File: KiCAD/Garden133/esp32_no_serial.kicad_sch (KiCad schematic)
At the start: 13 parts, among them J1 USB_B_Micro, J2 Edge2x6_Connector, U3 ESP32-WROOM-32, U4 NCP114ASN330T1G

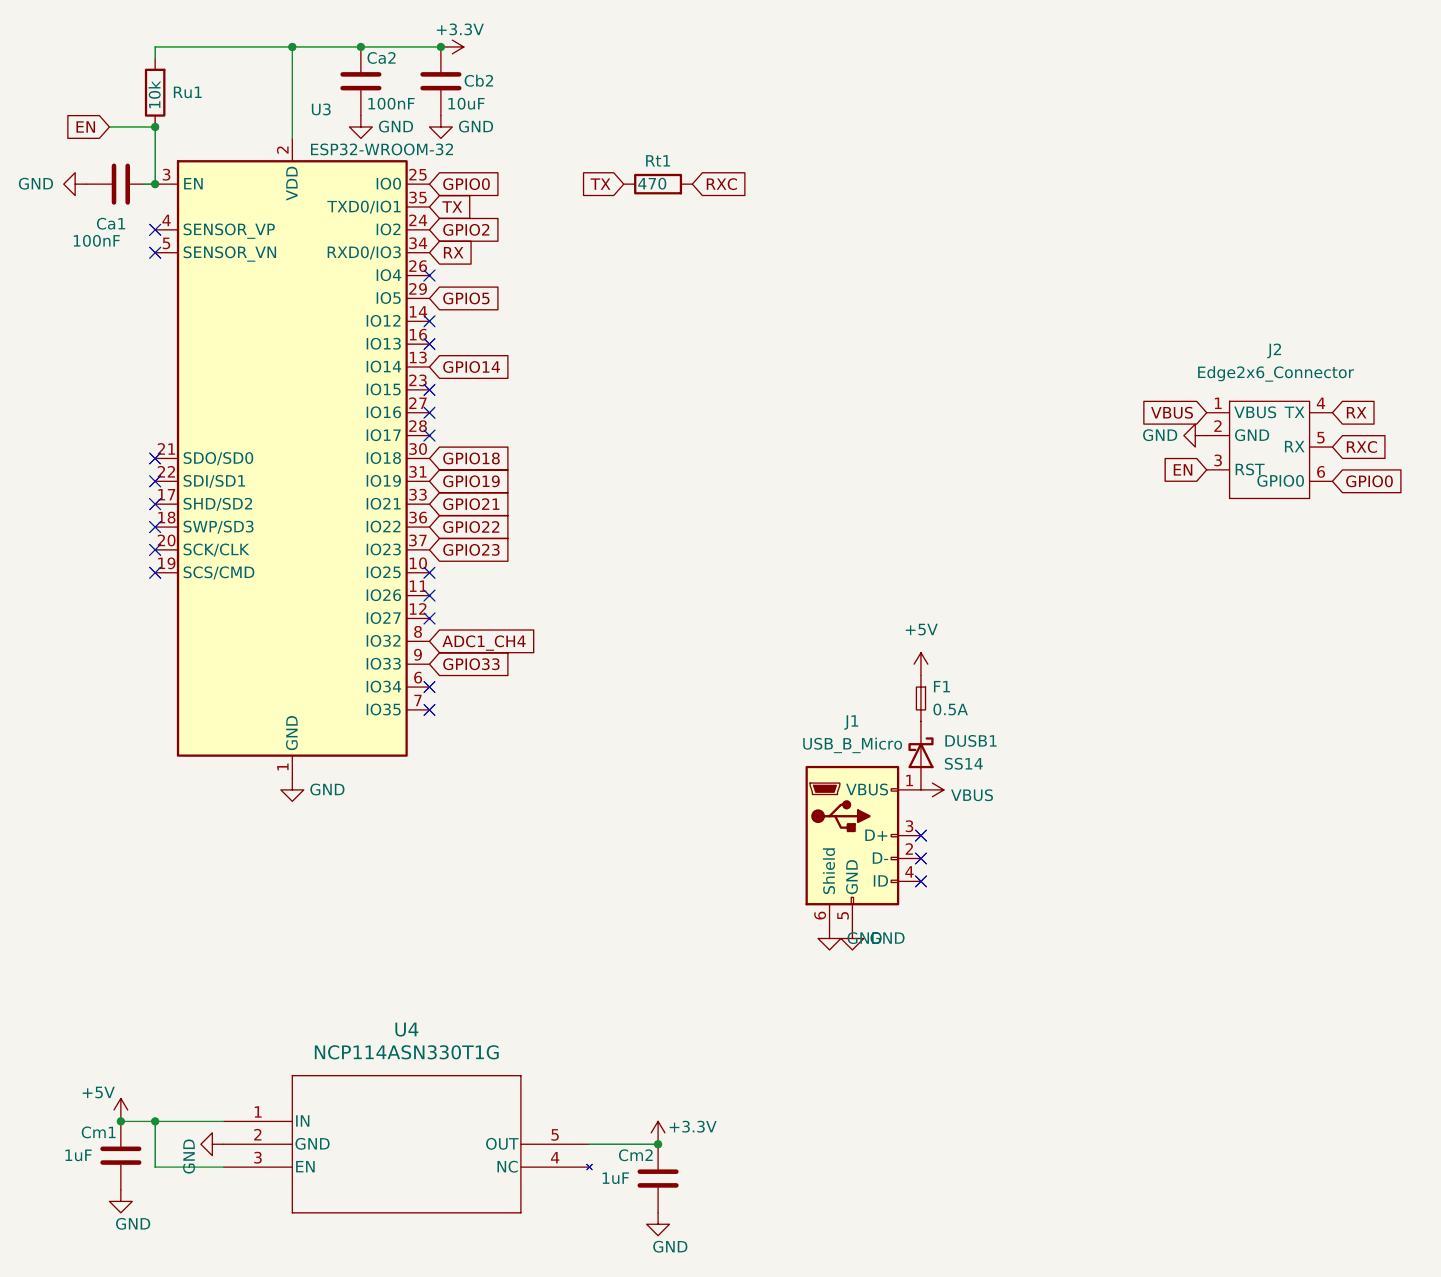
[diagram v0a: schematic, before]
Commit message: Board version 5
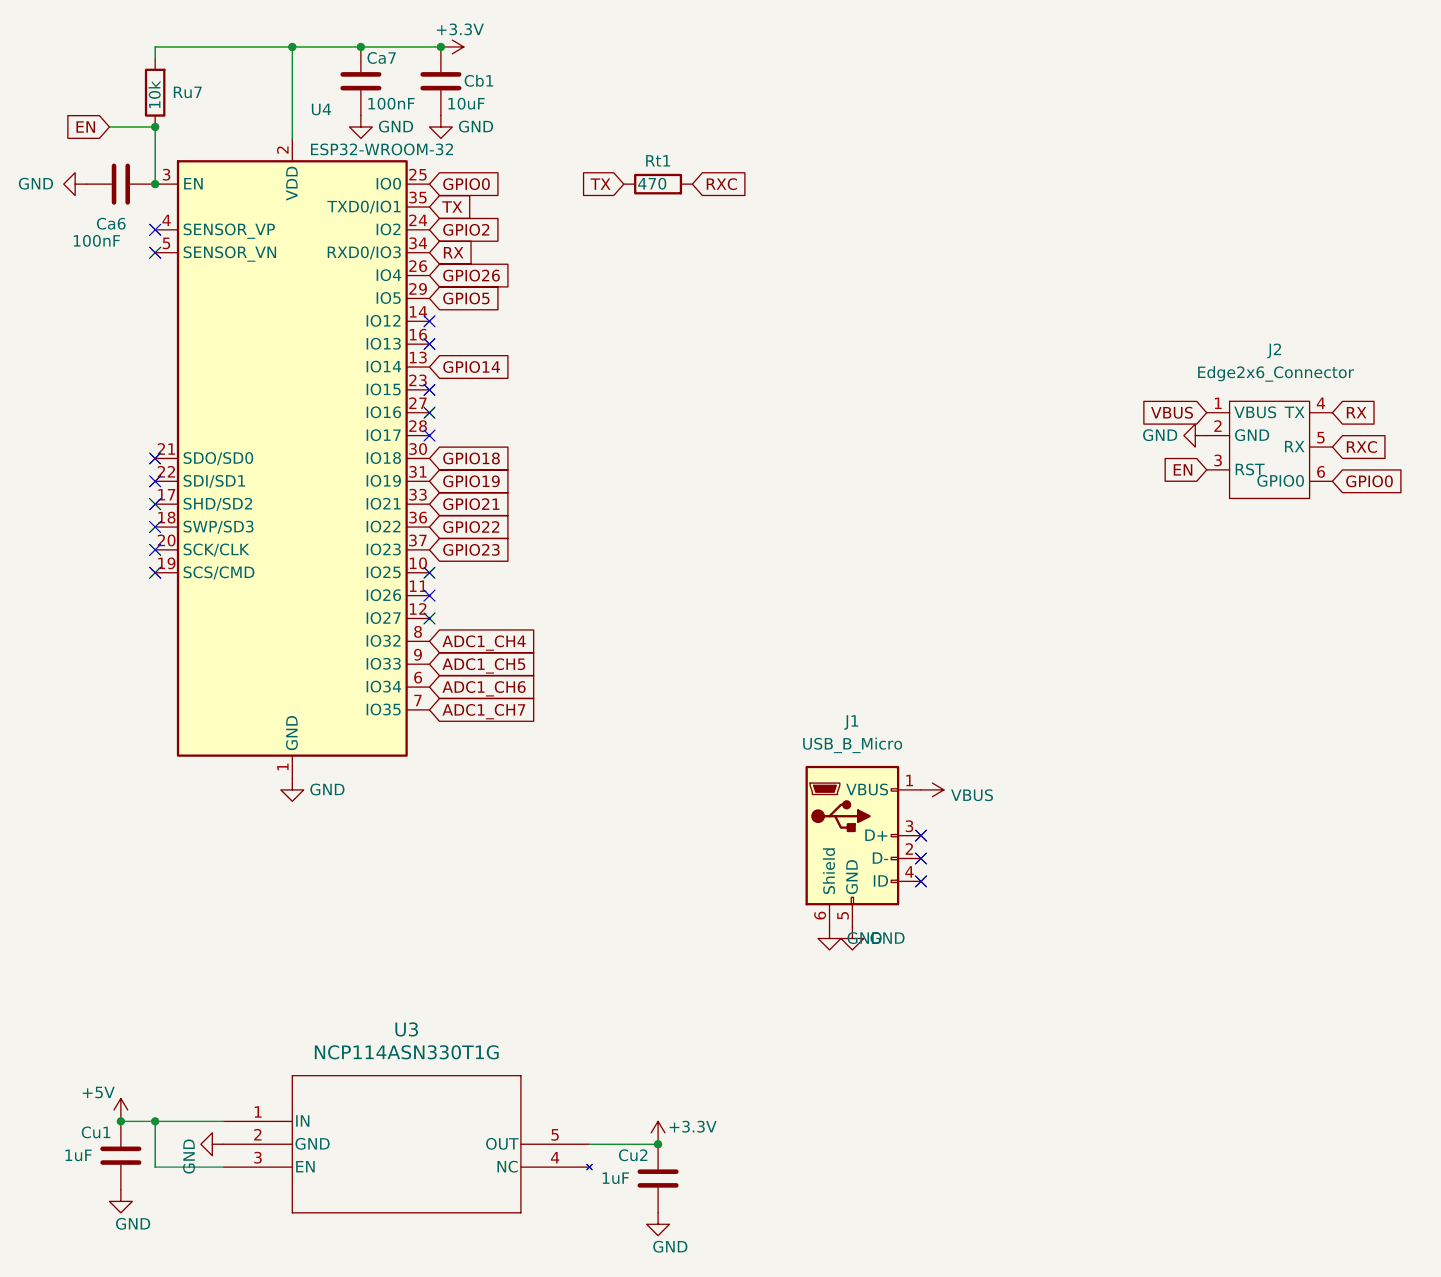
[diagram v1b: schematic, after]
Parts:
- removed DUSB1: SS14, Diode_SMD:D_2010_5025Metric, symbol Diode:1N5819
- removed F1: 0.5A, Diode_SMD:D_0805_2012Metric, symbol Device:Fuse_Small
- renumbered Ca1 to Ca6, Ca2 to Ca7, Cb2 to Cb1, Cm1 to Cu1, Cm2 to Cu2, Ru1 to Ru7, U4 to U3, U3 to U4
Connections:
- net GPIO26: now reaches U4.26 (IO4)
- net ADC1_CH6: now reaches U4.6 (IO34)
- net ADC1_CH7: now reaches U4.7 (IO35)
- net GPIO33 renamed ADC1_CH5
- no-connect marks 22 -> 19
